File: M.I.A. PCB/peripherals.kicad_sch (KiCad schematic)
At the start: 57 parts, among them J10 Conn_01x03, J11 Conn_01x03, J12 Screw_Terminal_01x02, J13 Screw_Terminal_01x02, J15 Screw_Terminal_01x02, J16 Screw_Terminal_01x02, J17 Screw_Terminal_01x02, J19 Conn_01x08_Socket, J20 Screw_Terminal_01x02, J21 Conn_01x04_Socket, J22 Conn_01x04_Socket, J3 Conn_01x03, J4 Conn_01x03, J5 Conn_01x03, J6 Conn_01x03, J7 MSD-4-A, J8 Conn_01x03, J9 Conn_01x03, Q1 AO3400A, Q2 AO3400A, Q3 AO3400A, Q4 AO3400A, U15 74AHC541

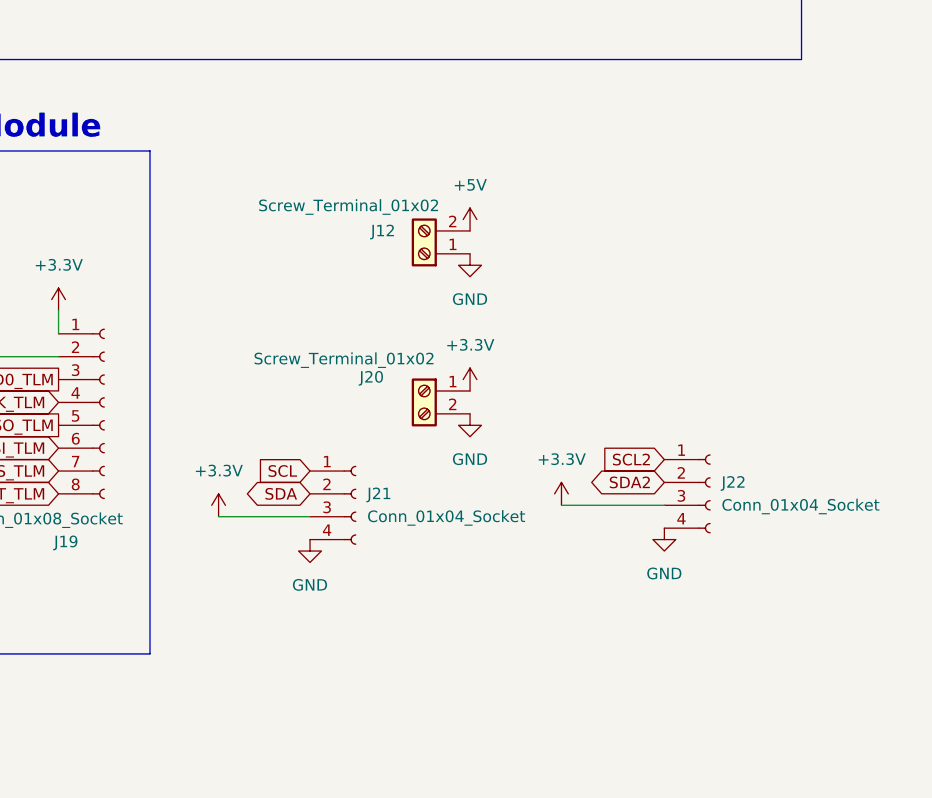
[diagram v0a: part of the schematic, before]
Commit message: Worked More on Layout/Wiring
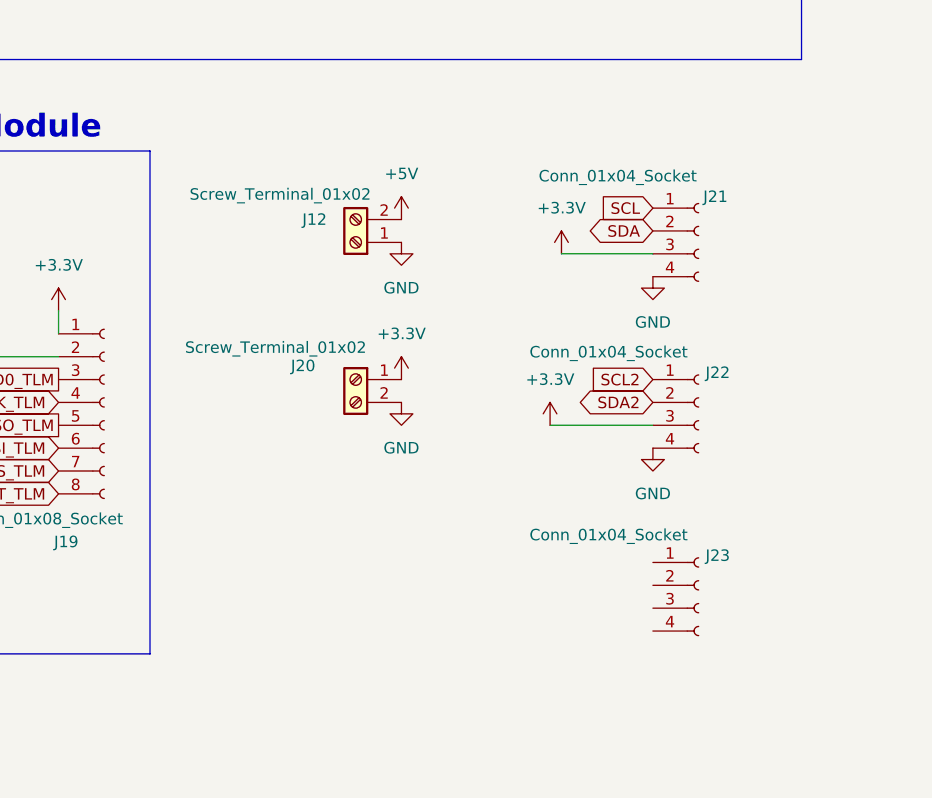
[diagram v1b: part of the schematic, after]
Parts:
- added J23: Conn_01x04_Socket, Connector_JST:JST_PH_B4B-PH-K_1x04_P2.00mm_Vertical, symbol Connector:Conn_01x04_Socket
- J12, J13, J15, J16, J17, J20: footprint TerminalBlock_Phoenix:TerminalBlock_Phoenix_PT-1,5-2-3.5-H_1x02_P3.50mm_Horizontal -> PCM_SparkFun-Connector:ScrewTerminal_1x02_P3.5mm_Horizontal_Black
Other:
- moved on the sheet: J12, J20, J21, J22
